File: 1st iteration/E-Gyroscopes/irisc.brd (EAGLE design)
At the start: 160 x 100 mm, 30 parts, among them Q3 FA-128, T1 BC846, U1 ANALOG_DEVICES_ADXRS646BBGZEV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, U11 LTC6655CHMS8-3.3PBF

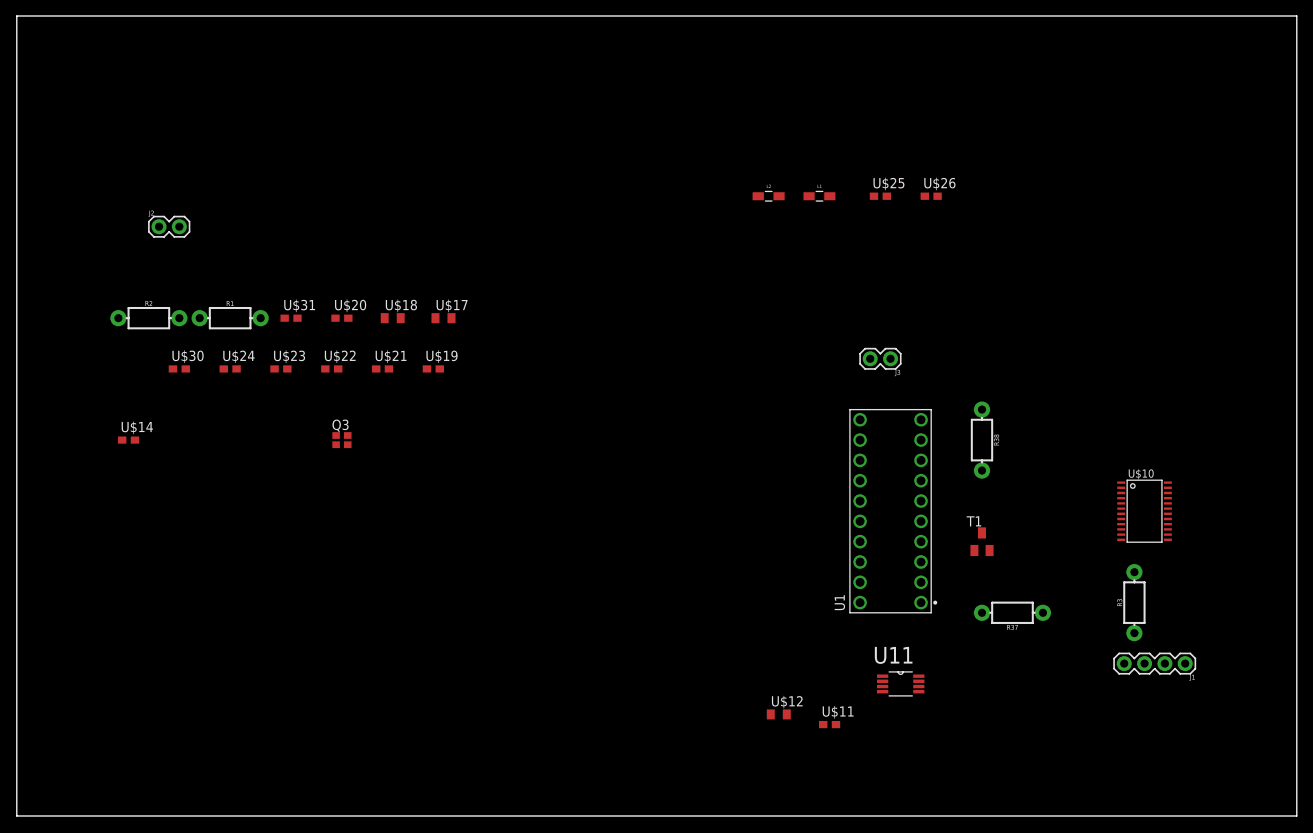
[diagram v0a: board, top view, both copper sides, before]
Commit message: Final E systems: schematics & PCB's
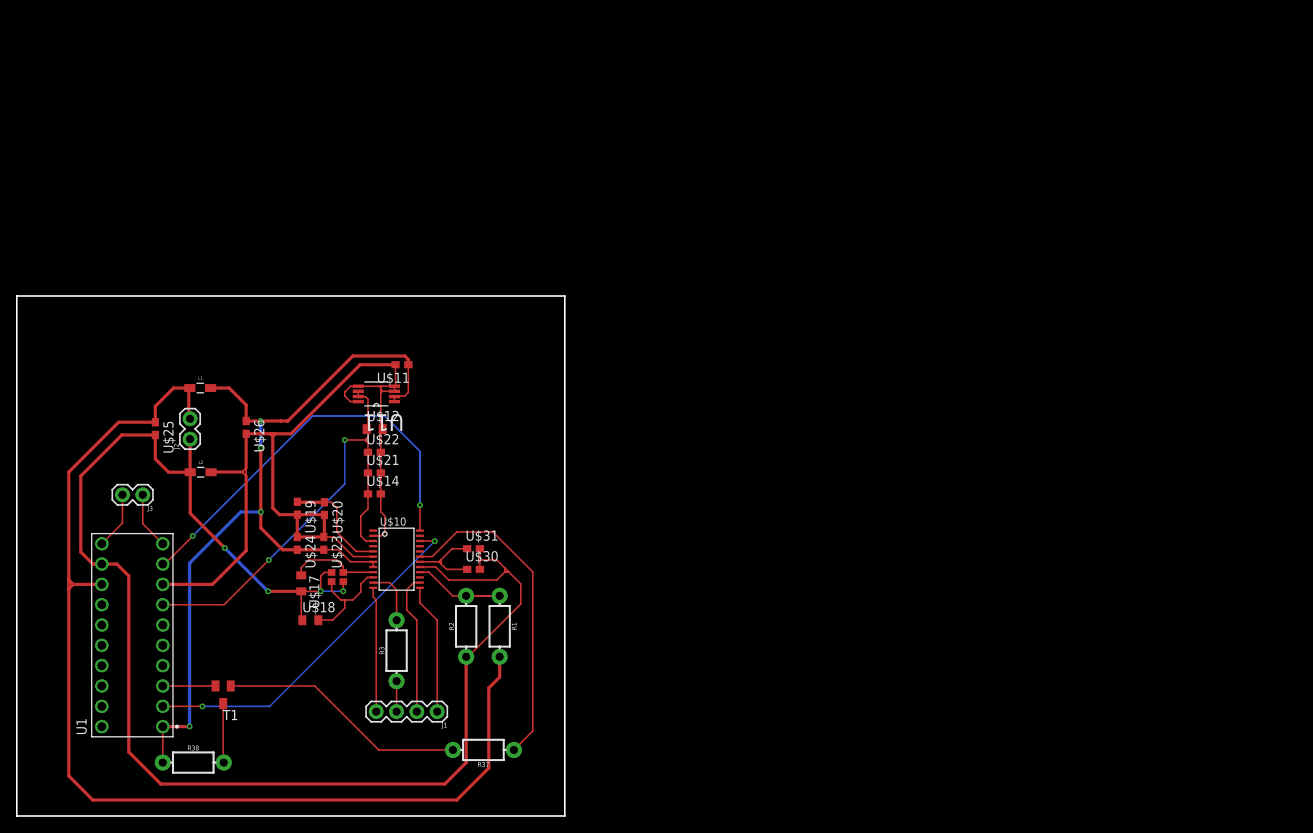
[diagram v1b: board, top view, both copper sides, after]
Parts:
- moved R38 106.5 mm to (22.1, 6.68), turned to 0 degrees
- moved T1 96.8 mm to (25.8, 15.2), turned to 180 degrees
- moved U1 96.0 mm to (18.2, 11.2)
- moved U$25 95.2 mm to (17.3, 48.4), turned to 270 degrees
- moved J3 95.0 mm to (15.8, 40.1)
- moved J1 93.7 mm to (52.5, 13.1)
- moved U$10 93.7 mm to (47.5, 32.1)
- moved R3 92.4 mm to (47.5, 20.7)
- moved U$26 90.4 mm to (28.7, 48.6), turned to 270 degrees
- moved L1 81.0 mm to (22.9, 53.5)
- moved L2 78.9 mm to (23.0, 43.0)
- moved U11 74.9 mm to (45.0, 52.8), turned to 180 degrees
- moved U$11 69.9 mm to (48.1, 56.4), turned to 180 degrees
- moved R37 68.3 mm to (58.3, 8.26)
- moved U$12 61.8 mm to (44.7, 48.4)
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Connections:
- net CS: now also J1.2; no longer J1.4
- net MOSI: now also J1.4; no longer J1.2
- net N$59: now also U$10.24; no longer U$10.21
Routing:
- net 0: track 0.00 -> 190.9 mm, vias 0 -> 4
- net 5V: track 0.00 -> 137.6 mm
- net GND: track 0.00 -> 121.9 mm
- net VCCA: track 0.00 -> 107.5 mm, vias 0 -> 4
- net N$48: track 0.00 -> 60.0 mm, vias 0 -> 2
- net N$59: track 0.00 -> 51.6 mm, vias 0 -> 2
- net N$58: track 0.00 -> 44.4 mm, vias 0 -> 2
- net N$66: track 0.00 -> 40.7 mm
- net N$46: track 0.00 -> 31.1 mm
- net CS: track 0.00 -> 17.8 mm
- net CLK: track 0.00 -> 16.4 mm
- net MOSI: track 0.00 -> 15.6 mm
- net N$50: track 0.00 -> 15.4 mm
- net N$45: track 0.00 -> 13.8 mm
- net N$2: track 0.00 -> 13.5 mm
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- added copper zone on layer 1, net 0
- added copper zone on layer 1, net 5V
- added copper zone on layer 1, net GND
- added copper zone on layer 1, net N$2
- added copper zone on layer 1, net N$48
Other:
- board size 160 x 100 mm -> 68.5 x 65 mm
